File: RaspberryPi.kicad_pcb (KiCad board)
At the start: 4 copper layers, 100 x 100 mm, 48 parts, among them P1 USB_C_Receptacle_Amphenol_124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, Q1 SO-8_3.9x4.9mm_P1.27mm, U1 SUP_TPS3831L30DQNR, U10 TFBGA453, U12 BGA96C80P6X16_900X1400X120, U13 BGA96C80P6X16_900X1400X120, U14 BGA96C80P6X16_900X1400X120, U15 BGA96C80P6X16_900X1400X120, U2 SOT-23-5_HandSoldering, U3 SOT-23-5, U4 VSSOP-10_3x3mm_P0.5mm, U5 SO-8_3.9x4.9mm_P1.27mm, U6 BGA-4_2x2_0.7x0.7mm

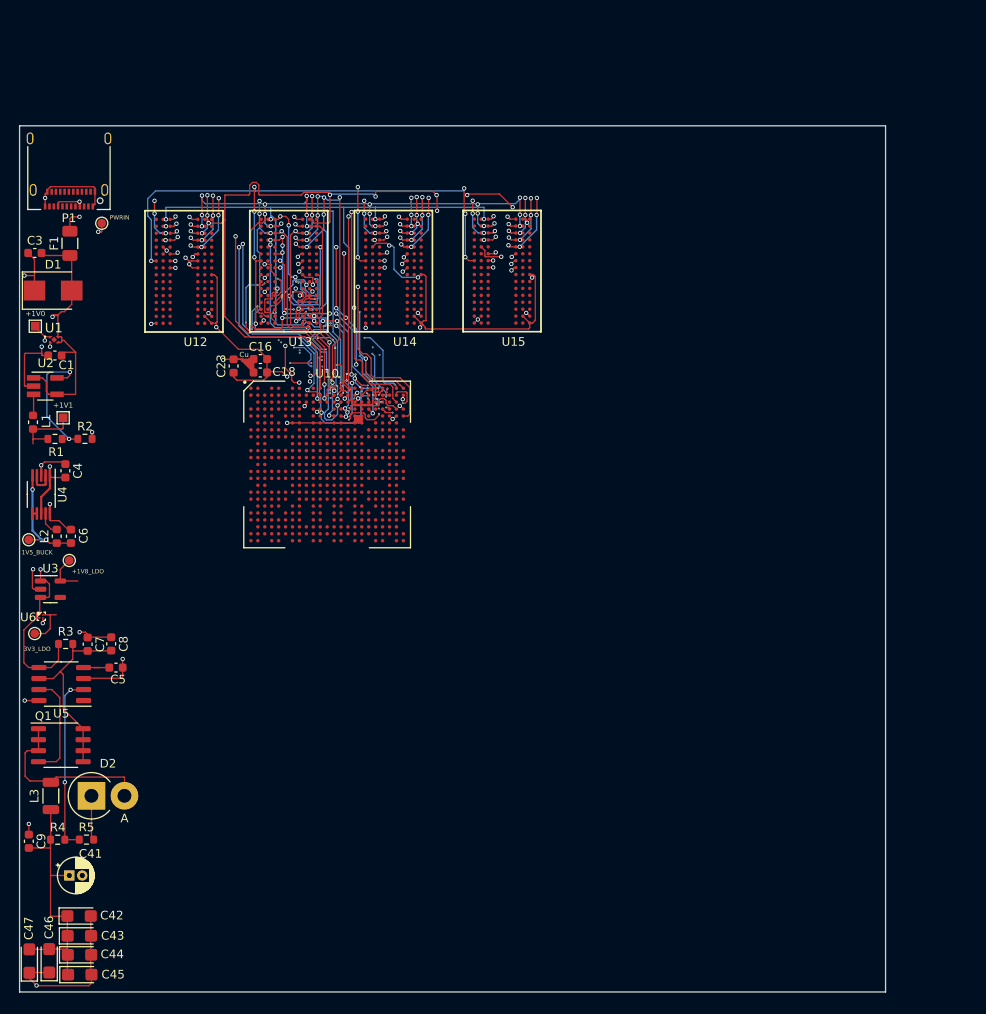
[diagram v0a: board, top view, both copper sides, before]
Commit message: 5-16 PC
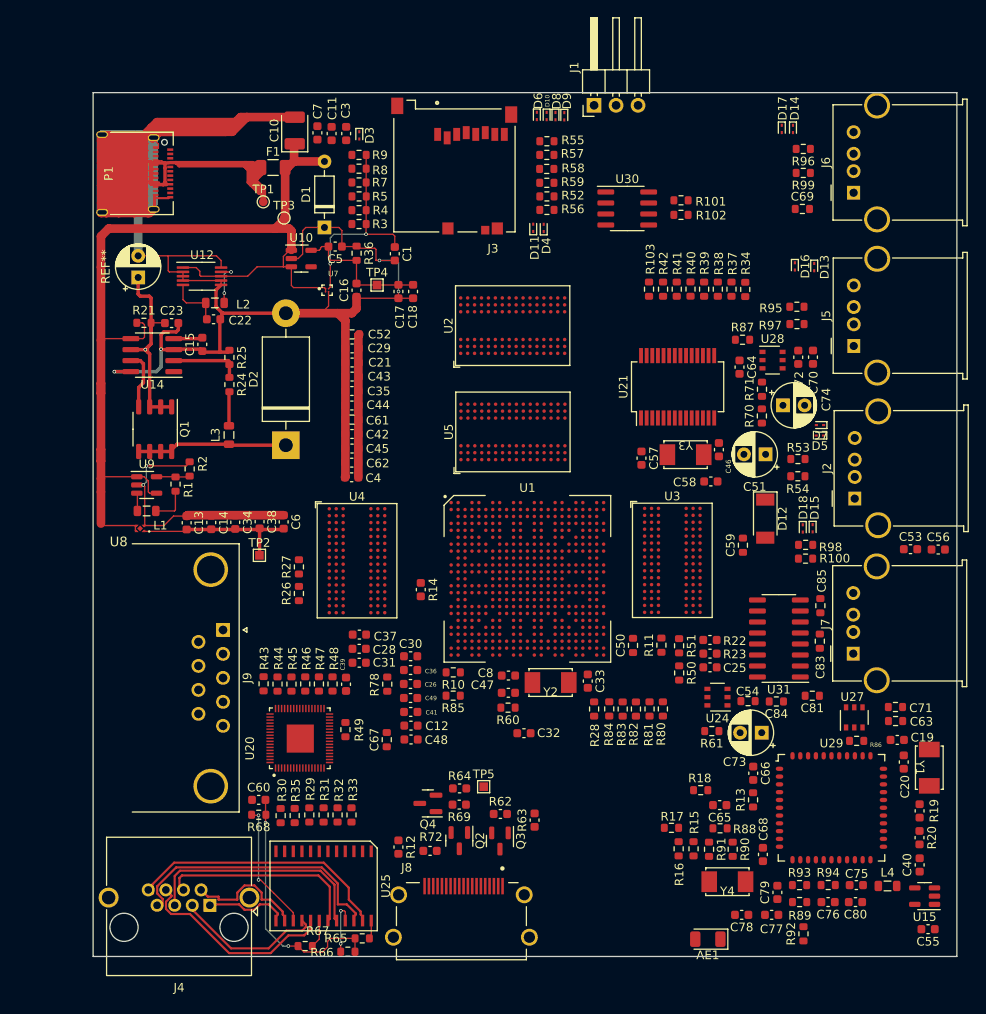
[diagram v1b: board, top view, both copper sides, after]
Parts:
- removed +1V0, +1V1: TestPoint_Pad_1.0x1.0mm, TestPoint:TestPoint_Pad_1.0x1.0mm
- removed +1V8_LDO, 1V5_BUCK, 3V3_LDO, PWRIN: TestPoint_Pad_D1.0mm, TestPoint:TestPoint_Pad_D1.0mm
- removed C9: C_0603_1608Metric, Capacitor_SMD:C_0603_1608Metric
- removed U13: BGA96C80P6X16_900X1400X120, symbols:BGA96C80P6X16_900X1400X120
- removed U6: BGA-4_2x2_0.7x0.7mm, Lib:BGA-4_2x2_0.7x0.7mm
- added AE1: Antenna, RF_Antenna:Johanson_2450AT18x100, F.Cu at (152.3, 147.2)
- added C10: 47uF, Capacitor_Tantalum_SMD:CP_EIA-3528-21_Kemet-B, F.Cu at (104.6, 53.8)
- added C11: 10uF, Capacitor_SMD:C_0603_1608Metric, F.Cu at (108.8, 54.2)
- added C12: 10uF, Capacitor_SMD:C_0603_1608Metric, F.Cu at (118.0, 122.5)
- added C13: 100nF, Capacitor_SMD:C_0603_1608Metric, F.Cu at (92.1, 99.1)
- added C14: 1nF, Capacitor_SMD:C_0603_1608Metric, F.Cu at (94.9, 99.1)
- added C15: 0.1uF, Capacitor_SMD:C_0603_1608Metric, F.Cu at (93.9, 78.5)
- added C17: 100nF, Capacitor_SMD:C_0603_1608Metric, F.Cu at (116.5, 72.4)
- added C19: 22pF, Capacitor_SMD:C_0603_1608Metric, F.Cu at (174.1, 124.2)
- added C20: 22pF, Capacitor_SMD:C_0603_1608Metric, F.Cu at (174.9, 126.7)
- added C21: 100nF, Capacitor_SMD:C_0603_1608Metric, F.Cu at (111.2, 80.6)
- added C22: 22uF, Capacitor_SMD:C_0603_1608Metric, F.Cu at (95.2, 75.6)
- added C25: 1nF, Capacitor_SMD:C_0603_1608Metric, F.Cu at (152.5, 115.8)
- added C26: 10nF, Capacitor_SMD:C_0603_1608Metric, F.Cu at (117.9, 117.7)
- added C28: 10nF, Capacitor_SMD:C_0603_1608Metric, F.Cu at (112.0, 113.7)
- added C29: 10uF, Capacitor_SMD:C_0603_1608Metric, F.Cu at (111.2, 79.0)
- added C30: 100nF, Capacitor_SMD:C_0603_1608Metric, F.Cu at (118.0, 114.5)
- added C31: 100nF, Capacitor_SMD:C_0603_1608Metric, F.Cu at (112.0, 115.3)
- added C32: 12pF, Capacitor_SMD:C_0603_1608Metric, F.Cu at (131.0, 123.4)
- added C33: 12pF, Capacitor_SMD:C_0603_1608Metric, F.Cu at (138.4, 117.4)
- added C34: 1uF, Capacitor_SMD:C_0603_1608Metric, F.Cu at (97.7, 99.0)
- added C35: 100nF, Capacitor_SMD:C_0603_1608Metric, F.Cu at (111.2, 83.9)
- added C36: 100nF, Capacitor_SMD:C_0603_1608Metric, F.Cu at (118.0, 116.1)
- added C37: 22uF, Capacitor_SMD:C_0603_1608Metric, F.Cu at (112.0, 112.0)
- added C38: 10nF, Capacitor_SMD:C_0603_1608Metric, F.Cu at (100.5, 99.0)
- added C39: 100nF, Capacitor_SMD:C_0603_1608Metric, F.Cu at (110.5, 117.8)
- added C40: 100nF, Capacitor_SMD:C_0603_1608Metric, F.Cu at (176.7, 138.6)
- added C48: 1uF, Capacitor_SMD:C_0603_1608Metric, F.Cu at (118.0, 124.1)
- added C49: 100nF, Capacitor_SMD:C_0603_1608Metric, F.Cu at (118.0, 119.3)
- added C50: 100nF, Resistor_SMD:R_0603_1608Metric, F.Cu at (143.6, 113.3)
- added C51: CP_Radial_D5.0mm_P2.50mm, Capacitor_THT:CP_Radial_D5.0mm_P2.50mm, F.Cu at (158.9, 91.2)
- added C52: 10uF, Resistor_SMD:R_0603_1608Metric, F.Cu at (111.2, 77.4)
- added C53: 100nF, Capacitor_SMD:C_0603_1608Metric, F.Cu at (175.7, 102.2)
- added C54: 100nF, Resistor_SMD:R_0603_1608Metric, F.Cu at (156.9, 119.7)
- added C55: 10nF, Capacitor_SMD:C_0603_1608Metric, F.Cu at (177.7, 146.0)
- added C56: 1uF, Capacitor_SMD:C_0603_1608Metric, F.Cu at (178.9, 102.2)
- added C57: 22pF, Capacitor_SMD:C_0603_1608Metric, F.Cu at (144.6, 91.7)
- added C58: 22pF, Capacitor_SMD:C_0603_1608Metric, F.Cu at (152.6, 94.3)
- added C59: 10uF, Resistor_SMD:R_0603_1608Metric, F.Cu at (156.3, 101.7)
- added C60: 1nF, Capacitor_SMD:C_0603_1608Metric, F.Cu at (100.4, 131.1)
- added C61: 10uF, Resistor_SMD:R_0603_1608Metric, F.Cu at (111.2, 87.2)
- added C62: 10uF, Capacitor_SMD:C_0603_1608Metric, F.Cu at (111.2, 92.2)
- added C63: 100nF, Resistor_SMD:R_0603_1608Metric, F.Cu at (173.9, 122.0)
- added C64: 100nF, Capacitor_SMD:C_0603_1608Metric, F.Cu at (155.9, 81.1)
- added C65: 18pF, Capacitor_SMD:C_0603_1608Metric, F.Cu at (153.6, 131.7)
- added C66: 10pF, Capacitor_SMD:C_0603_1608Metric, F.Cu at (157.5, 128.0)
- added C67: 22pF, Resistor_SMD:R_0603_1608Metric, F.Cu at (115.2, 124.2)
- added C68: 18pF, Capacitor_SMD:C_0603_1608Metric, F.Cu at (158.6, 137.4)
- added C69: 10uF, Resistor_SMD:R_0603_1608Metric, F.Cu at (163.2, 62.9)
- added C70: 10uF, Capacitor_SMD:C_0603_1608Metric, F.Cu at (164.4, 80.0)
- added C71: 0.1uF, Resistor_SMD:R_0603_1608Metric, F.Cu at (173.9, 120.4)
- added C72: 0.1uF, Capacitor_SMD:C_0603_1608Metric, F.Cu at (162.7, 80.0)
- added C73: CP_Radial_D5.0mm_P2.50mm, Capacitor_THT:CP_Radial_D5.0mm_P2.50mm, F.Cu at (158.5, 123.3)
- added C74: CP_Radial_D5.0mm_P2.50mm, Capacitor_THT:CP_Radial_D5.0mm_P2.50mm, F.Cu at (160.9, 85.5)
- added C75: 18pF, Capacitor_SMD:C_0603_1608Metric, F.Cu at (169.4, 140.9)
- added C76: 18pF, Capacitor_SMD:C_0603_1608Metric, F.Cu at (166.2, 142.9)
- added C77: 18pF, Capacitor_SMD:C_0603_1608Metric, F.Cu at (159.6, 144.4)
- added C78: 18pF, Capacitor_SMD:C_0603_1608Metric, F.Cu at (156.2, 144.4)
- added C79: 18pF, Capacitor_SMD:C_0603_1608Metric, F.Cu at (160.3, 141.8)
- added C80: 18pF, Capacitor_SMD:C_0603_1608Metric, F.Cu at (169.3, 142.9)
- added C81: 100nF, Resistor_SMD:R_0603_1608Metric, F.Cu at (164.3, 119.1)
- added C83: 100nF, Resistor_SMD:R_0603_1608Metric, F.Cu at (165.2, 112.8)
- added C84: 100nF, Resistor_SMD:R_0603_1608Metric, F.Cu at (160.2, 119.7)
- added C85: 100nF, Resistor_SMD:R_0603_1608Metric, F.Cu at (165.3, 108.7)
- added D10: ESD9B5VL, Diode_SMD:D_SOD-923, F.Cu at (133.7, 52.1)
- added D11: ESD9B5VL, Diode_SMD:D_SOD-923, F.Cu at (132.1, 65.1)
- added D12: PMEG3030BEP, Diode_SMD:D_SOD-128, F.Cu at (158.9, 98.6)
- added D13: ESD9B5VL, Diode_SMD:D_SOD-923, F.Cu at (164.6, 69.6)
- added D14: ESD9B5VL, Diode_SMD:D_SOD-923, F.Cu at (162.1, 53.6)
- added D15: ESD9B5VL, Diode_SMD:D_SOD-923, F.Cu at (164.4, 99.7)
- added D16: ESD9B5VL, Diode_SMD:D_SOD-923, F.Cu at (162.3, 69.5)
- added D17: ESD9B5VL, Diode_SMD:D_SOD-923, F.Cu at (160.8, 53.6)
- added D18: ESD9B5VL, Diode_SMD:D_SOD-923, F.Cu at (163.2, 99.8)
- added D3: ESD9B5VL, Diode_SMD:D_SOD-923, F.Cu at (112.0, 54.4)
- added D4: ESD9B5VL, Diode_SMD:D_SOD-923, F.Cu at (133.3, 65.1)
- added D5: ESD9B5VL, Diode_SMD:D_SOD-923, F.Cu at (165.2, 89.0)
- added D6: ESD9B5VL, Diode_SMD:D_SOD-923, F.Cu at (132.5, 52.1)
- added D7: ESD9B5VL, Diode_SMD:D_SOD-923, F.Cu at (165.2, 87.8)
- added D8: ESD9B5VL, Diode_SMD:D_SOD-923, F.Cu at (134.7, 52.2)
- added D9: ESD9B5VL, Diode_SMD:D_SOD-923, F.Cu at (135.7, 52.2)
- added J1: DBG1, Connector_PinHeader_2.54mm:PinHeader_1x03_P2.54mm_Horizontal, F.Cu at (139.1, 50.9)
- added J2: USB_A, Connector_USB:USB_A_Molex_67643_Horizontal, F.Cu at (169.2, 96.3)
- added J3: Micro_SD_Card_Det, symbols:MOLEX_47352-1001, F.Cu at (123.0, 57.9)
- added J4: RJ45, Connector_RJ:RJ45_Amphenol_RJHSE5380, F.Cu at (94.8, 143.3)
- added J5: USB_A, Connector_USB:USB_A_Molex_67643_Horizontal, F.Cu at (169.1, 78.7)
- added J6: USB_A, Connector_USB:USB_A_Molex_67643_Horizontal, F.Cu at (169.1, 61.0)
- added J7: USB_A, Connector_USB:USB_A_Molex_67643_Horizontal, F.Cu at (169.1, 114.2)
- added J8: HDMI_A, symbols:AMPHENOL_10029449-001RLF, F.Cu at (123.8, 142.1)
- added J9: DB9_Male, Connector_Dsub:DSUB-9_Male_Horizontal_P2.77x2.84mm_EdgePinOffset7.70mm_Housed_MountingHolesOffset9.12mm, F.Cu at (96.3, 111.5)
- added L4: 3.3uH, Inductor_SMD:L_0805_2012Metric, F.Cu at (173.0, 141.0)
- added Q2: 2N7002, Package_TO_SOT_SMD:SOT-23, F.Cu at (123.6, 135.8)
- added Q3: 2N7002, Package_TO_SOT_SMD:SOT-23, F.Cu at (128.3, 135.8)
- added Q4: 2N7002, Package_TO_SOT_SMD:SOT-23, F.Cu at (120.0, 131.5)
- added R10: 10K, Resistor_SMD:R_0603_1608Metric, F.Cu at (122.9, 116.4)
- added R100: 90, Resistor_SMD:R_0603_1608Metric, F.Cu at (163.6, 103.2)
- added R101: 10K, Resistor_SMD:R_0603_1608Metric, F.Cu at (149.2, 61.9)
- added R102: 2.2K, Resistor_SMD:R_0603_1608Metric, F.Cu at (149.2, 63.6)
- added R103: 2.2K, Resistor_SMD:R_0603_1608Metric, F.Cu at (145.5, 72.1)
- added R11: 133R, Resistor_SMD:R_0603_1608Metric, F.Cu at (146.9, 113.2)
- added R12: 1K, Capacitor_SMD:C_0603_1608Metric, F.Cu at (116.5, 136.6)
- added R13: 10K, Resistor_SMD:R_0603_1608Metric, F.Cu at (157.5, 131.1)
- added R14: 1.62K, Capacitor_SMD:C_0603_1608Metric, F.Cu at (119.1, 106.8)
- added R15: 10K, Resistor_SMD:R_0603_1608Metric, F.Cu at (150.6, 136.8)
- added R16: 10K, Resistor_SMD:R_0603_1608Metric, F.Cu at (148.9, 136.8)
- added R17: 10K, Resistor_SMD:R_0603_1608Metric, F.Cu at (148.1, 134.3)
- added R18: 10K, Resistor_SMD:R_0603_1608Metric, F.Cu at (151.4, 130.0)
- added R19: 10K, Capacitor_SMD:C_0603_1608Metric, F.Cu at (176.7, 132.4)
- added R20: 22R, Capacitor_SMD:C_0603_1608Metric, F.Cu at (176.7, 135.5)
- added R21: 0.05R, Resistor_SMD:R_0603_1608Metric, F.Cu at (87.2, 76.0)
- added R22: 1K, Capacitor_SMD:C_0603_1608Metric, F.Cu at (152.5, 112.6)
- added R23: 1K, Capacitor_SMD:C_0603_1608Metric, F.Cu at (152.5, 114.2)
- added R24: 180K, Resistor_SMD:R_0603_1608Metric, F.Cu at (97.0, 83.2)
- added R25: 150K, Resistor_SMD:R_0603_1608Metric, F.Cu at (97.0, 80.0)
- added R26: 6.8K, Resistor_SMD:R_0603_1608Metric, F.Cu at (105.1, 107.3)
- added R27: 10K, Resistor_SMD:R_0603_1608Metric, F.Cu at (105.1, 104.2)
- added R28: 1M, Resistor_SMD:R_0603_1608Metric, F.Cu at (139.1, 120.6)
- added R29: 4K7, Resistor_SMD:R_0603_1608Metric, F.Cu at (106.3, 132.8)
- added R30: 4K7, Resistor_SMD:R_0603_1608Metric, F.Cu at (103.0, 132.9)
- added R31: 4K7, Resistor_SMD:R_0603_1608Metric, F.Cu at (107.9, 132.8)
- added R32: 4K7, Resistor_SMD:R_0603_1608Metric, F.Cu at (109.5, 132.8)
- added R33: 4K7, Resistor_SMD:R_0603_1608Metric, F.Cu at (111.1, 132.8)
- added R34: 10K, Resistor_SMD:R_0603_1608Metric, F.Cu at (156.6, 72.2)
- added R35: 4K7, Resistor_SMD:R_0603_1608Metric, F.Cu at (104.6, 132.9)
- added R36: 510R, Resistor_SMD:R_0603_1608Metric, F.Cu at (111.7, 68.0)
- added R37: 680R, Resistor_SMD:R_0603_1608Metric, F.Cu at (155.0, 72.1)
- added R38: 10K, Resistor_SMD:R_0603_1608Metric, F.Cu at (153.4, 72.1)
- added R39: 10K, Resistor_SMD:R_0603_1608Metric, F.Cu at (151.8, 72.1)
- added R40: 100K, Resistor_SMD:R_0603_1608Metric, F.Cu at (150.3, 72.1)
- added R41: 10K, Resistor_SMD:R_0603_1608Metric, F.Cu at (148.7, 72.1)
- added R42: 10K, Resistor_SMD:R_0603_1608Metric, F.Cu at (147.1, 72.1)
- added R43: 2.49K, Resistor_SMD:R_0603_1608Metric, F.Cu at (101.0, 117.7)
- added R44: 4K7, Resistor_SMD:R_0603_1608Metric, F.Cu at (102.6, 117.7)
- added R45: 4K7, Resistor_SMD:R_0603_1608Metric, F.Cu at (104.2, 117.7)
- added R46: 4K7, Resistor_SMD:R_0603_1608Metric, F.Cu at (105.8, 117.7)
- added R47: 4K7, Resistor_SMD:R_0603_1608Metric, F.Cu at (107.4, 117.7)
- added R48: 1K5, Resistor_SMD:R_0603_1608Metric, F.Cu at (108.9, 117.7)
- added R49: 4K7, Resistor_SMD:R_0603_1608Metric, F.Cu at (110.4, 123.0)
- added R50: 10K, Resistor_SMD:R_0603_1608Metric, F.Cu at (149.0, 116.5)
- added R51: 15K, Resistor_SMD:R_0603_1608Metric, F.Cu at (148.9, 113.3)
- added R52: 22R, Resistor_SMD:R_0603_1608Metric, F.Cu at (133.7, 61.4)
- added R53: 90, Resistor_SMD:R_0603_1608Metric, F.Cu at (162.7, 91.8)
- added R54: 90, Resistor_SMD:R_0603_1608Metric, F.Cu at (162.7, 93.7)
- added R55: 22R, Resistor_SMD:R_0603_1608Metric, F.Cu at (133.7, 55.1)
- added R56: 22R, Resistor_SMD:R_0603_1608Metric, F.Cu at (133.7, 63.0)
- added R57: 22R, Resistor_SMD:R_0603_1608Metric, F.Cu at (133.7, 56.6)
- added R58: 22R, Resistor_SMD:R_0603_1608Metric, F.Cu at (133.7, 58.3)
- added R59: 22R, Resistor_SMD:R_0603_1608Metric, F.Cu at (133.7, 59.9)
- added R60: 10K, Resistor_SMD:R_0603_1608Metric, F.Cu at (129.2, 120.5)
- added R61: 20K, Resistor_SMD:R_0603_1608Metric, F.Cu at (152.7, 123.2)
- added R62: 10K, Capacitor_SMD:C_0603_1608Metric, F.Cu at (128.3, 132.7)
- added R63: 4.7K, Capacitor_SMD:C_0603_1608Metric, F.Cu at (132.3, 133.4)
- added R64: 4.7K, Capacitor_SMD:C_0603_1608Metric, F.Cu at (123.6, 129.8)
- added R65: 75, Resistor_SMD:R_0603_1608Metric, F.Cu at (112.4, 147.1)
- added R66: 75, Resistor_SMD:R_0603_1608Metric, F.Cu at (110.7, 148.6)
- added R67: 75, Resistor_SMD:R_0603_1608Metric, F.Cu at (105.8, 148.0)
- added R68: 75, Resistor_SMD:R_0603_1608Metric, F.Cu at (100.4, 132.8)
- added R69: 1.5K, Capacitor_SMD:C_0603_1608Metric, F.Cu at (123.6, 131.7)
- added R7: 10K, Resistor_SMD:R_0603_1608Metric, F.Cu at (112.0, 59.8)
- added R70: 10K, Resistor_SMD:R_0603_1608Metric, F.Cu at (158.5, 86.8)
- added R71: 10K, Resistor_SMD:R_0603_1608Metric, F.Cu at (158.5, 83.7)
- added R72: 1.5K, Capacitor_SMD:C_0603_1608Metric, F.Cu at (120.2, 137.0)
- added R78: 22, Resistor_SMD:R_0603_1608Metric, F.Cu at (115.3, 117.7)
- added R8: 10K, Resistor_SMD:R_0603_1608Metric, F.Cu at (112.0, 58.2)
- added R80: 22, Resistor_SMD:R_0603_1608Metric, F.Cu at (147.1, 120.6)
- added R81: 22, Resistor_SMD:R_0603_1608Metric, F.Cu at (145.5, 120.6)
- added R82: 22, Resistor_SMD:R_0603_1608Metric, F.Cu at (144.0, 120.6)
- added R83: 22, Resistor_SMD:R_0603_1608Metric, F.Cu at (142.4, 120.6)
- added R84: 22, Resistor_SMD:R_0603_1608Metric, F.Cu at (140.9, 120.6)
- added R85: 22, Resistor_SMD:R_0603_1608Metric, F.Cu at (122.9, 119.1)
- added R86: 20K, Resistor_SMD:R_0603_1608Metric, F.Cu at (169.4, 124.3)
- added R87: 20K, Resistor_SMD:R_0603_1608Metric, F.Cu at (156.3, 78.0)
- added R88: 100R, Resistor_SMD:R_0603_1608Metric, F.Cu at (153.7, 134.4)
- added R89: 22R, Resistor_SMD:R_0603_1608Metric, F.Cu at (162.9, 142.9)
- added R9: 10K, Resistor_SMD:R_0603_1608Metric, F.Cu at (112.0, 56.6)
- added R90: 22R, Resistor_SMD:R_0603_1608Metric, F.Cu at (155.1, 136.8)
- added R91: 22R, Resistor_SMD:R_0603_1608Metric, F.Cu at (152.4, 136.8)
- added R92: 22R, Resistor_SMD:R_0603_1608Metric, F.Cu at (163.3, 146.6)
- added R93: 22R, Resistor_SMD:R_0603_1608Metric, F.Cu at (162.9, 140.9)
- added R94: 22R, Resistor_SMD:R_0603_1608Metric, F.Cu at (166.2, 140.9)
- added R95: 90, Resistor_SMD:R_0603_1608Metric, F.Cu at (162.6, 74.2)
- added R96: 90, Resistor_SMD:R_0603_1608Metric, F.Cu at (163.3, 56.0)
- added R97: 90, Resistor_SMD:R_0603_1608Metric, F.Cu at (162.6, 76.2)
- added R98: 90, Resistor_SMD:R_0603_1608Metric, F.Cu at (163.6, 101.7)
- added R99: 90, Resistor_SMD:R_0603_1608Metric, F.Cu at (163.3, 58.7)
- added REF**: CP_Radial_D5.0mm_P2.50mm, Capacitor_THT:CP_Radial_D5.0mm_P2.50mm, F.Cu at (86.5, 70.8)
- added TP1: +5, TestPoint:TestPoint_Pad_D1.0mm, F.Cu at (100.9, 62.1)
- added TP2: 1V_USB, TestPoint:TestPoint_Pad_1.0x1.0mm, F.Cu at (100.5, 102.9)
- added TP3: +5, TestPoint:TestPoint_Pad_D1.0mm, F.Cu at (103.3, 63.9)
- added TP4: 1V8_USB, TestPoint:TestPoint_Pad_1.0x1.0mm, F.Cu at (114.1, 71.7)
- added TP5: 3V3_IO, TestPoint:TestPoint_Pad_1.0x1.0mm, F.Cu at (126.4, 129.6)
- added U20: RTL8211E-VB-CG, symbols:QFN35P700X700X80-69N, F.Cu at (105.2, 124.0)
- added U21: GL852G, Package_SO:SSOP-28_5.3x10.2mm_P0.65mm, F.Cu at (148.8, 83.4)
- added U24: MP65151DJ, Package_SO:TSOP-6_1.65x3.05mm_P0.95mm, F.Cu at (153.4, 119.2)
- added U25: GST5009, Library:SOIC-24, F.Cu at (107.9, 141.0)
- added U27: MP65151DJ, Package_SO:TSOP-6_1.65x3.05mm_P0.95mm, F.Cu at (169.2, 121.6)
- added U28: MP65151DJ, Package_SO:TSOP-6_1.65x3.05mm_P0.95mm, F.Cu at (159.7, 80.3)
- added U29: AP6335, Library:AP6335, F.Cu at (166.5, 132.0)
- added U30: AT24C16B, Package_SO:SOIC-8_3.9x4.9mm_P1.27mm, F.Cu at (143.0, 62.8)
- added U31: MAX3232, Package_SO:SOIC-16_3.9x9.9mm_P1.27mm, F.Cu at (160.5, 112.5)
- added U7: TPS7A21, symbols:BGA4N35P2X2_64X64X33, F.Cu at (108.3, 72.3)
- added U8: TPS7A0310, symbols:SUP_TPS3831L30DQNR, F.Cu at (86.7, 99.8)
- added U9: TLV62565-LibCool, Package_TO_SOT_SMD:SOT-23-5, F.Cu at (87.5, 94.7)
- added Y1: 32.768kHz, Library:OSC_5032, F.Cu at (176.2, 127.4)
- added Y2: 24MHz, Library:OSC_5032, F.Cu at (134.1, 119.2)
- added Y3: 12MHz, Library:OSC_5032, F.Cu at (149.7, 89.6)
- added Y4: 37.4MHz, Library:OSC_5032, F.Cu at (154.5, 142.1)
- C1, C23, C4, C5, C6: value C_0603_1608Metric -> 100nF
- C16: value C_0603_1608Metric -> 10uF
- C18, C8: value C_0603_1608Metric -> 10nF
- C3: value C_0603_1608Metric -> 1uF
- C41: value CP_Radial_D4.0mm_P1.50mm -> 1nF; footprint Capacitor_THT:CP_Radial_D4.0mm_P1.50mm -> Capacitor_SMD:C_0603_1608Metric
- C42, C43, C44, C45, C47: value CP_EIA-3216-18_Kemet-A -> 100nF; footprint Capacitor_Tantalum_SMD:CP_EIA-3216-18_Kemet-A -> Capacitor_SMD:C_0603_1608Metric
- C46: value CP_EIA-3216-18_Kemet-A -> 1uF; footprint Capacitor_Tantalum_SMD:CP_EIA-3216-18_Kemet-A -> Capacitor_SMD:C_0603_1608Metric
- C7: value C_0603_1608Metric -> 4.7uF
- D1: value D_SMB -> SMBJ5.0A; footprint Diode_SMD:D_SMB -> Diode_THT:D_DO-35_SOD27_P7.62mm_Horizontal
- D2: value D_DO-201AD_P3.81mm_Vertical_AnodeUp -> 1N5820; footprint Diode_THT:D_DO-201AD_P3.81mm_Vertical_AnodeUp -> Diode_THT:D_DO-201AD_P15.24mm_Horizontal
- F1: value Fuse_1206_3216Metric -> 5A
- L1: value L_0603_1608Metric -> 2.2uH; footprint Inductor_SMD:L_0603_1608Metric -> Inductor_SMD:L_0805_2012Metric
- L2: value L_0603_1608Metric -> 10uH; footprint Inductor_SMD:L_0603_1608Metric -> Inductor_SMD:L_0805_2012Metric
- L3: value L_1206_3216Metric -> 47uH; footprint Inductor_SMD:L_1206_3216Metric -> Inductor_SMD:L_0805_2012Metric
- P1: value USB_C_Receptacle_Amphenol_12401610E4-2A -> USB_C_Plug_USB2.0
- Q1: value SO-8_3.9x4.9mm_P1.27mm -> Si9430
- R1: value R_0603_1608Metric -> 100K
- R2: value R_0603_1608Metric -> 120K
- R3, R4, R5: value R_0603_1608Metric -> 10K
- U1: value SUP_TPS3831L30DQNR -> RK3368; footprint symbols:SUP_TPS3831L30DQNR -> Library:TFBGA453
- U10: value TFBGA453 -> TPS72118; footprint Lib:TFBGA453 -> Package_TO_SOT_SMD:SOT-23-5
- U12: value BGA96C80P6X16_900X1400X120 -> TPS62052DGS; footprint symbols:BGA96C80P6X16_900X1400X120 -> Package_SO:VSSOP-10_3x3mm_P0.5mm
- U14: value BGA96C80P6X16_900X1400X120 -> MAX1651; footprint symbols:BGA96C80P6X16_900X1400X120 -> Package_SO:SOIC-8_3.9x4.9mm_P1.27mm
- U15: value BGA96C80P6X16_900X1400X120 -> SN74LVC1G14DBV; footprint symbols:BGA96C80P6X16_900X1400X120 -> Package_TO_SOT_SMD:SOT-23-5
- U2: value SOT-23-5_HandSoldering -> MT41KxxxM16TW; footprint Package_TO_SOT_SMD:SOT-23-5_HandSoldering -> Package_BGA:BGA-96_9.0x13.0mm_Layout2x3x16_P0.8mm
- U3: value SOT-23-5 -> MT41KxxxM16TW; footprint Package_TO_SOT_SMD:SOT-23-5 -> Package_BGA:BGA-96_9.0x13.0mm_Layout2x3x16_P0.8mm
- U4: value VSSOP-10_3x3mm_P0.5mm -> MT41KxxxM16TW; footprint Package_SO:VSSOP-10_3x3mm_P0.5mm -> Package_BGA:BGA-96_9.0x13.0mm_Layout2x3x16_P0.8mm
- U5: value SO-8_3.9x4.9mm_P1.27mm -> MT41KxxxM16TW; footprint Package_SO:SO-8_3.9x4.9mm_P1.27mm -> Package_BGA:BGA-96_9.0x13.0mm_Layout2x3x16_P0.8mm
- moved C46 97.3 mm to (153.6, 90.7)
- moved U15 87.1 mm to (177.3, 142.2)
- moved R5 80.7 mm to (112.0, 61.4)
- moved R4 80.6 mm to (112.0, 63.0)
- moved U3 71.9 mm to (148.2, 103.5)
- moved C43 71.8 mm to (111.2, 82.2)
- moved C44 70.8 mm to (111.2, 85.6)
- moved C45 68.4 mm to (111.2, 90.5)
- moved C7 64.7 mm to (107.2, 54.1)
- moved C42 64.0 mm to (111.2, 88.9)
- moved C47 63.4 mm to (129.2, 118.7), turned to 0 degrees
- moved U1 61.2 mm to (131.4, 105.6)
- moved U5 59.7 mm to (129.8, 88.6), turned to 90 degrees
- moved R3 59.1 mm to (112.0, 64.6)
- moved C5 54.8 mm to (109.2, 67.2), turned to 180 degrees
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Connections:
- C1 pad 1: (no net) -> +3.3VP
- C1 pad 2: +5V -> GND
- C16 pad 1: (no net) -> GND
- C16 pad 2: (no net) -> +1V8
- C18 pad 1: (no net) -> GND
- C18 pad 2: (no net) -> +1V8
- C23 pad 1: (no net) -> Net-(Q1-S)
- C23 pad 2: (no net) -> GND
- C3 pad 1: (no net) -> +5V
- C3 pad 2: +5V -> GND
- C4 pad 1: (no net) -> GND
- C4 pad 2: +5V -> +3V3
- C41 pad 1: +3V3 -> GND
- C41 pad 2: (no net) -> +1V0
- C42 pad 1: +3V3 -> GND
- C42 pad 2: (no net) -> +3V3
- C43 pad 1: +3V3 -> GND
- C43 pad 2: (no net) -> +3V3
- C44 pad 1: +3V3 -> GND
- C44 pad 2: (no net) -> +3V3
- C45 pad 1: +3V3 -> GND
- C45 pad 2: (no net) -> +3V3
- C46 pad 1: (no net) -> GND
- C46 pad 2: +3V3 -> Net-(U21-RESET#)
- C47 pad 1: (no net) -> /RST
- C47 pad 2: +3V3 -> GND
- C5 pad 1: (no net) -> GND
- C5 pad 2: (no net) -> +1V8
- C6 pad 1: +1V5 -> GND
- C6 pad 2: (no net) -> +1V0
- C7 pad 1: (no net) -> GND
- C7 pad 2: (no net) -> +5V
- C8 pad 1: (no net) -> GND
- C8 pad 2: (no net) -> /RECOVER
- D1 pad 1: (no net) -> GND
- D2 pad 1: (no net) -> Net-(D2-K)
- D2 pad 2: (no net) -> GND
- F1 pad 1: +5V -> Net-(P1-VBUS)
- F1 pad 2: PWRIN -> +5V
- L1 pad 1: (no net) -> +1V1
- L1 pad 2: (no net) -> Net-(U9-SW)
- L2 pad 1: +1V5 -> Net-(U12-SW)
- L2 pad 2: (no net) -> +1V5
- L3 pad 1: +3V3 -> Net-(D2-K)
- L3 pad 2: (no net) -> +3V3
- P1 pad A1: (no net) -> GND
- P1 pad A12: (no net) -> GND
- P1 pad A4: PWRIN -> Net-(P1-VBUS)
- P1 pad A5: (no net) -> unconnected-(P1-CC)
- P1 pad A6: (no net) -> unconnected-(P1-D+)
- P1 pad A7: (no net) -> unconnected-(P1-D-)
- P1 pad A9: PWRIN -> Net-(P1-VBUS)
- P1 pad B1: (no net) -> GND
- P1 pad B12: (no net) -> GND
- P1 pad B4: (no net) -> Net-(P1-VBUS)
- P1 pad B5: (no net) -> unconnected-(P1-VCONN)
- P1 pad B9: (no net) -> Net-(P1-VBUS)
- P1 pad S1: (no net) -> GND
- Q1 pad 1: (no net) -> Net-(Q1-S)
- Q1 pad 2: (no net) -> Net-(Q1-S)
- Q1 pad 3: (no net) -> Net-(Q1-S)
- Q1 pad 4: (no net) -> Net-(Q1-G)
- Q1 pad 5: (no net) -> Net-(D2-K)
- Q1 pad 6: (no net) -> Net-(D2-K)
- Q1 pad 7: (no net) -> Net-(D2-K)
- Q1 pad 8: (no net) -> Net-(D2-K)
- R1 pad 1: (no net) -> Net-(U9-FB)
- R1 pad 2: 1V1FB -> +1V1
- R2 pad 1: (no net) -> GND
- R2 pad 2: (no net) -> Net-(U9-FB)
- R3 pad 1: +5V -> /SDMMC_D0
- R3 pad 2: (no net) -> +3.3VP
- R4 pad 1: +3V3 -> /SDMMC_D1
- R4 pad 2: (no net) -> +3.3VP
- R5 pad 1: (no net) -> /SDMMC_D2
- R5 pad 2: (no net) -> +3.3VP
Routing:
- net (no net): track 2518.0 -> 0.00 mm, vias 340 -> 0
- net GND: track 511.8 -> 431.0 mm, vias 42 -> 6
- net Net-(P1-VBUS): track 0.00 -> 66.8 mm
- net +5V: track 89.1 -> 126.4 mm, vias 3 -> 0
- net TD1-: track 0.00 -> 31.4 mm
- net TD1+: track 0.00 -> 31.2 mm
- net Net-(C60-Pad2): track 0.00 -> 28.9 mm, vias 0 -> 2
- net TD2+: track 0.00 -> 27.0 mm
- net Net-(Q1-S): track 0.00 -> 24.9 mm, vias 0 -> 1
- net +3.3VP: track 0.00 -> 24.1 mm, vias 0 -> 2
- net TD3+: track 0.00 -> 23.6 mm
- net TD2-: track 0.00 -> 23.6 mm
- net Net-(D2-K): track 0.00 -> 17.5 mm
- net TD3-: track 0.00 -> 17.4 mm
- net +1V0: track 2.74 -> 19.4 mm, vias 1 -> 0
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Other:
- board size 100 x 100 mm -> 99.7 x 99.7 mm
- board text removed: "Cu"
